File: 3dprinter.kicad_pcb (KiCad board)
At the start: 2 copper layers, 148.1 x 75 mm, 111 parts, among them J1 6P IDC CONNECTOR, J10 MCU_PROG, J11 Conn_01x04, J12 MCU_PROG, J13 Conn_01x04, J14 MCU_PROG, J15 Conn_01x04, J16 MCU_PROG, J17 Conn_02x04_Odd_Even, J18 Conn_01x18, J2 USB_B_Micro, J3 Conn_01x02, J4 X_END, J5 Thermistor, J6 Y_END, J7 Z_END, J8 Heaters & Fans, J9 Conn_01x04, Q1 Mos, Q2 Mos, Q3 Mos, SW1 6x6 SMD, U1 ATmega2560-16A, U2 FT232RL, U3 L7805, Y1 16MHz

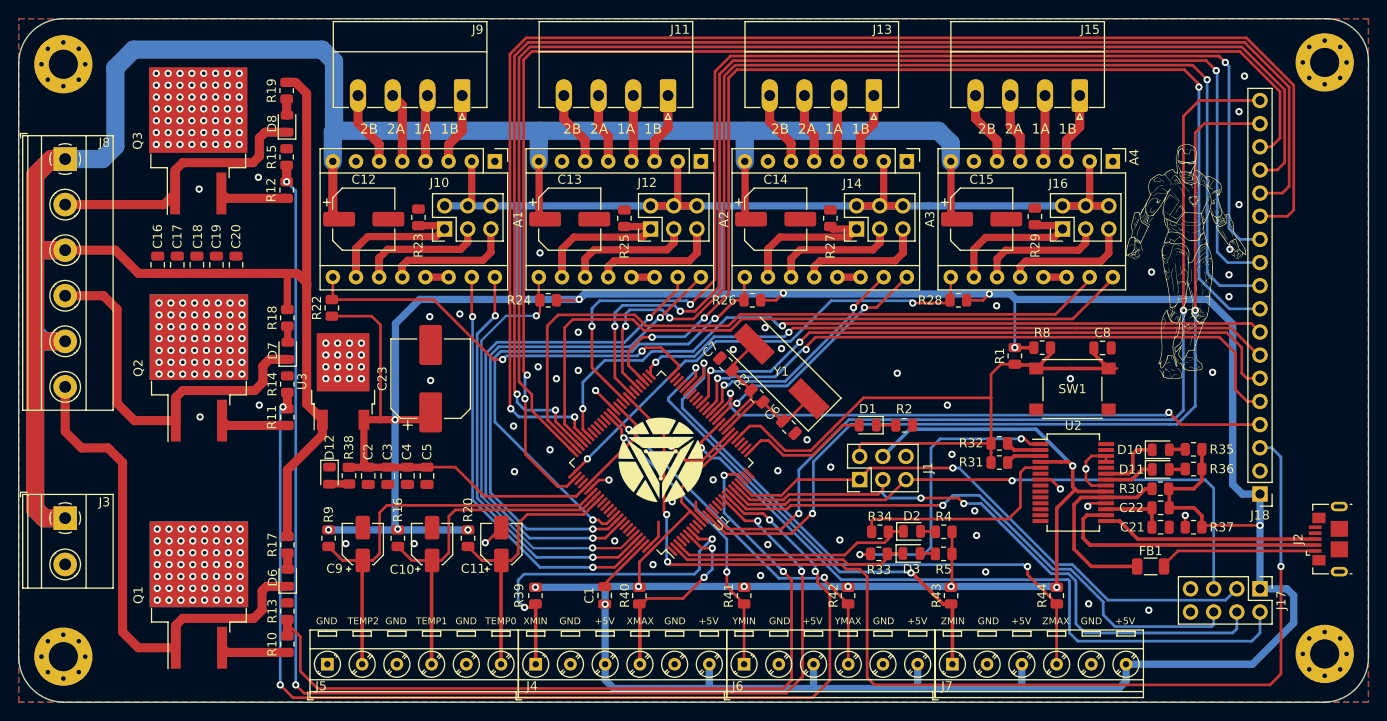
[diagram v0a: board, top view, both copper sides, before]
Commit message: LAST
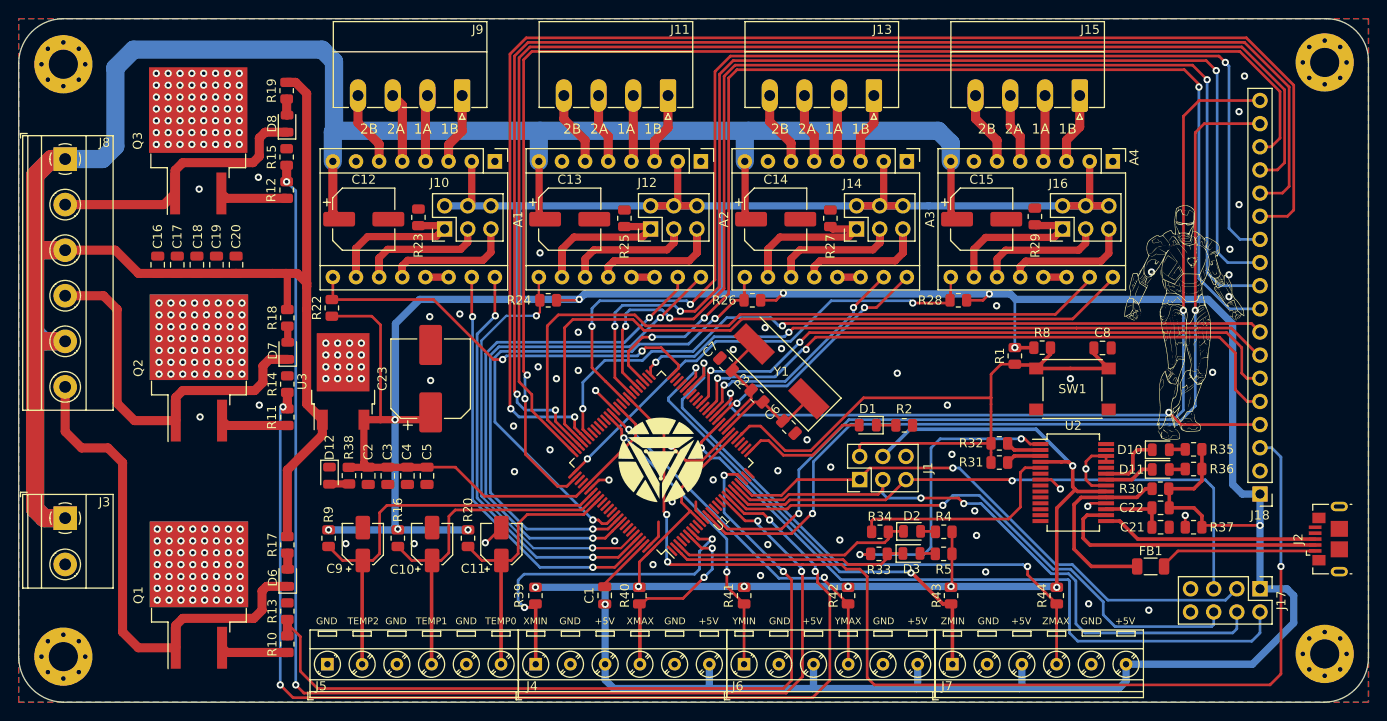
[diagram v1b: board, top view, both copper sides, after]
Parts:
- moved G*** 6.70 mm to (230.2, 80.4)
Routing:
- net Y_EN: track 49.5 -> 48.3 mm
- net THERM1: track 40.0 -> 39.0 mm
- net RES: track 77.2 -> 76.3 mm
- net D37: track 124.0 -> 123.3 mm
